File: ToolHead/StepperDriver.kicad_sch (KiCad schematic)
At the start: 1 part, among them J9 Conn_01x04

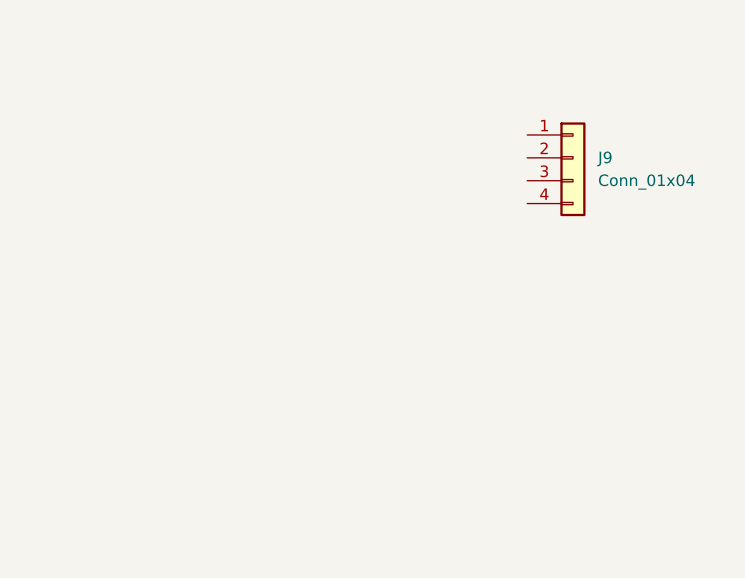
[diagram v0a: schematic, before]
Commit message: Moderate update. Moving to other computer.
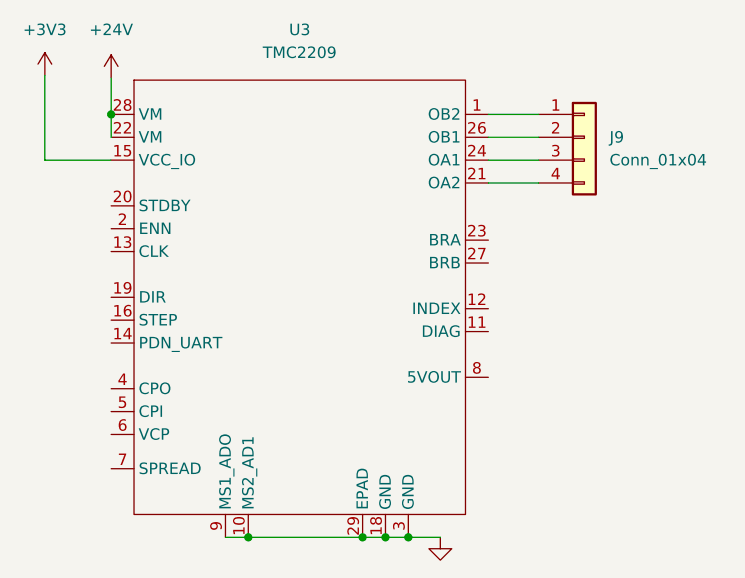
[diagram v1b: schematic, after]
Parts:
- added U3: TMC2209, Package_DFN_QFN:QFN-28-1EP_5x5mm_P0.5mm_EP3.75x3.75mm_ThermalVias, symbol Custom:TMC2209
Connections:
- net at J9.1 (Pin_1): now also U3.1 (OB2)
- net at J9.2 (Pin_2): now also U3.26 (OB1)
- net at J9.3 (Pin_3): now also U3.24 (OA1)
- net at J9.4 (Pin_4): now also U3.21 (OA2)
- new net +24V: U3.22 (VM), U3.28 (VM)
- new net +3V3: U3.15 (VCC_IO)
- new net GND: U3.10 (MS2_AD1), U3.18 (GND), U3.29 (EPAD), U3.3 (GND), U3.9 (MS1_ADO)
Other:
- moved on the sheet: J9
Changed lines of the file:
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@@
 (kicad_sch (version 20211123) (generator eeschema)
   (paper "A4")
-  (symbol (lib_id "Connector_Generic:Conn_01x04") (at 102.616 44.704 0) (unit 1)
+  (junction (at 66.548 86.868) (diameter 0) (color 0 0 0 0)
+  )
+  (junction (at 81.788 86.868) (diameter 0) (color 0 0 0 0)
+  )
+  (junction (at 79.248 86.868) (diameter 0) (color 0 0 0 0)
+  )
+  (junction (at 51.308 39.878) (diameter 0) (color 0 0 0 0)
+  )
+  (junction (at 84.328 86.868) (diameter 0) (color 0 0 0 0)
+  )
+  (wire (pts (xy 93.218 47.498) (xy 98.806 47.498))
+    (stroke (width 0) (type default) (color 0 0 0 0))
+  )
+  (wire (pts (xy 79.248 86.868) (xy 81.788 86.868))
+    (stroke (width 0) (type default) (color 0 0 0 0))
+  )
+  (wire (pts (xy 93.218 42.418) (xy 98.806 42.418))
+    (stroke (width 0) (type default) (color 0 0 0 0))
+  )
+  (wire (pts (xy 43.942 44.958) (xy 51.308 44.958))
+    (stroke (width 0) (type default) (color 0 0 0 0))
+  )
+  (wire (pts (xy 51.308 39.878) (xy 51.308 42.418))
+    (stroke (width 0) (type default) (color 0 0 0 0))
+  )
+  (wire (pts (xy 93.218 44.958) (xy 98.806 44.958))
+    (stroke (width 0) (type default) (color 0 0 0 0))
+  )
+  (wire (pts (xy 93.218 39.878) (xy 98.806 39.878))
+    (stroke (width 0) (type default) (color 0 0 0 0))
+  )
+  (wire (pts (xy 66.548 86.868) (xy 79.248 86.868))
+    (stroke (width 0) (type default) (color 0 0 0 0))
+  )
+  (wire (pts (xy 81.788 86.868) (xy 84.328 86.868))
+    (stroke (width 0) (type default) (color 0 0 0 0))
+  )
+  (wire (pts (xy 43.942 35.56) (xy 43.942 44.958))
+    (stroke (width 0) (type default) (color 0 0 0 0))
+  )
+  (wire (pts (xy 84.328 86.868) (xy 87.884 86.868))
+    (stroke (width 0) (type default) (color 0 0 0 0))
+  )
+  (wire (pts (xy 51.308 35.814) (xy 51.308 39.878))
+    (stroke (width 0) (type default) (color 0 0 0 0))
+  )
+  (wire (pts (xy 64.008 86.868) (xy 66.548 86.868))
+    (stroke (width 0) (type default) (color 0 0 0 0))
+  )
+  (symbol (lib_id "power:GND") (at 87.884 86.868 0) (unit 1)
     (in_bom yes) (on_board yes) (fields_autoplaced)
-    (property "Reference" "J9" (id 0) (at 105.41 44.7039 0)
+    (property "Reference" "#PWR0118" (id 0) (at 87.884 93.218 0)
+      (effects (font (size 1.27 1.27)) hide)
+    )
+    (property "Value" "GND" (id 1) (at 87.884 91.44 0)
+      (effects (font (size 1.27 1.27)) hide)
+    )
+    (property "Footprint" "" (id 2) (at 87.884 86.868 0)
+      (effects (font (size 1.27 1.27)) hide)
+    )
+    (property "Datasheet" "" (id 3) (at 87.884 86.868 0)
+      (effects (font (size 1.27 1.27)) hide)
+    )
+    (pin "1")
+  )
+  (symbol (lib_id "power:+3V3") (at 43.942 35.56 0) (unit 1)
+    (in_bom yes) (on_board yes) (fields_autoplaced)
+    (property "Reference" "#PWR0120" (id 0) (at 43.942 39.37 0)
+      (effects (font (size 1.27 1.27)) hide)
+    )
+    (property "Value" "+3V3" (id 1) (at 43.942 30.48 0))
+    (property "Footprint" "" (id 2) (at 43.942 35.56 0)
+      (effects (font (size 1.27 1.27)) hide)
+    )
+    (property "Datasheet" "" (id 3) (at 43.942 35.56 0)
+      (effects (font (size 1.27 1.27)) hide)
+    )
+    (pin "1")
+  )
+  (symbol (lib_id "Custom:TMC2209") (at 72.898 30.988 0) (unit 1)
+    (in_bom yes) (on_board yes) (fields_autoplaced)
+    (property "Reference" "U3" (id 0) (at 72.263 30.48 0))
+    (property "Value" "TMC2209" (id 1) (at 72.263 33.02 0))
+    (property "Footprint" "Package_DFN_QFN:QFN-28-1EP_5x5mm_P0.5mm_EP3.75x3.75mm_ThermalVias" (id 2) (at 72.898 30.988 0)
+      (effects (font (size 1.27 1.27)) hide)
+    )
+    (property "Datasheet" "" (id 3) (at 72.898 30.988 0)
+      (effects (font (size 1.27 1.27)) hide)
+    )
+    (pin "1")
+    (pin "10")
+    (pin "11")
+    (pin "12")
+    (pin "13")
+    (pin "14")
+    (pin "15")
+    (pin "16")
+    (pin "18")
+    (pin "19")
+    (pin "2")
+    (pin "20")
+    (pin "21")
+    (pin "22")
+    (pin "23")
+    (pin "24")
+    (pin "26")
+    (pin "27")
+    (pin "28")
+    (pin "29")
+    (pin "3")
+    (pin "4")
+    (pin "5")
+    (pin "6")
+    (pin "7")
+    (pin "8")
+    (pin "9")
+  )
+  (symbol (lib_id "power:+24V") (at 51.308 35.814 0) (unit 1)
+    (in_bom yes) (on_board yes) (fields_autoplaced)
+    (property "Reference" "#PWR0119" (id 0) (at 51.308 39.624 0)
+      (effects (font (size 1.27 1.27)) hide)
+    )
+    (property "Value" "+24V" (id 1) (at 51.308 30.48 0))
+    (property "Footprint" "" (id 2) (at 51.308 35.814 0)
+      (effects (font (size 1.27 1.27)) hide)
+    )
+    (property "Datasheet" "" (id 3) (at 51.308 35.814 0)
+      (effects (font (size 1.27 1.27)) hide)
+    )
+    (pin "1")
+  )
+  (symbol (lib_id "Connector_Generic:Conn_01x04") (at 103.886 42.418 0) (unit 1)
+    (in_bom yes) (on_board yes) (fields_autoplaced)
+    (property "Reference" "J9" (id 0) (at 106.68 42.4179 0)
       (effects (font (size 1.27 1.27)) (justify left))
     )
-    (property "Value" "Conn_01x04" (id 1) (at 105.41 47.2439 0)
+    (property "Value" "Conn_01x04" (id 1) (at 106.68 44.9579 0)
       (effects (font (size 1.27 1.27)) (justify left))
     )
-    (property "Footprint" "Connector_JST:JST_XH_S4B-XH-A-1_1x04_P2.50mm_Horizontal" (id 2) (at 102.616 44.704 0)
+    (property "Footprint" "Connector_JST:JST_XH_S4B-XH-A-1_1x04_P2.50mm_Horizontal" (id 2) (at 103.886 42.418 0)
       (effects (font (size 1.27 1.27)) hide)
     )
-    (property "Datasheet" "~" (id 3) (at 102.616 44.704 0)
+    (property "Datasheet" "~" (id 3) (at 103.886 42.418 0)
       (effects (font (size 1.27 1.27)) hide)
     )
